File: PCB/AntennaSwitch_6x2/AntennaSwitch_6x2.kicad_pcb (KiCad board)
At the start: 2 copper layers, 100 x 100 mm, 160 parts, among them J1 Conn_01x08, J2 Conn_01x08, J3 Conn_01x08, J4 HR913550A, J5 SWD, J6 485, J7 12VDC, J8 Conn_01x01, Q1 2N7002K, SW1 LOAD, SW2 SRBV170501, SW3 SRBV170501, SW4 M/R, SW5 RESET, U1 74HC238, U10 74HC148, U11 74HC148, U12 4511, U13 4511, U14 Blue 0.59'', U15 Blue 0.59'', U16 STM32F030F4Px, U17 MAX485E, U18 CH395Q, U19 AZ1117-1.8, U2 74HC573, U20 SY8303, U3 74HC573, U4 74HC238, U5 74HC00, U6 74HC00, U7 74HC00, U8 74HC04, U9 TLC555, Y1 30MHz

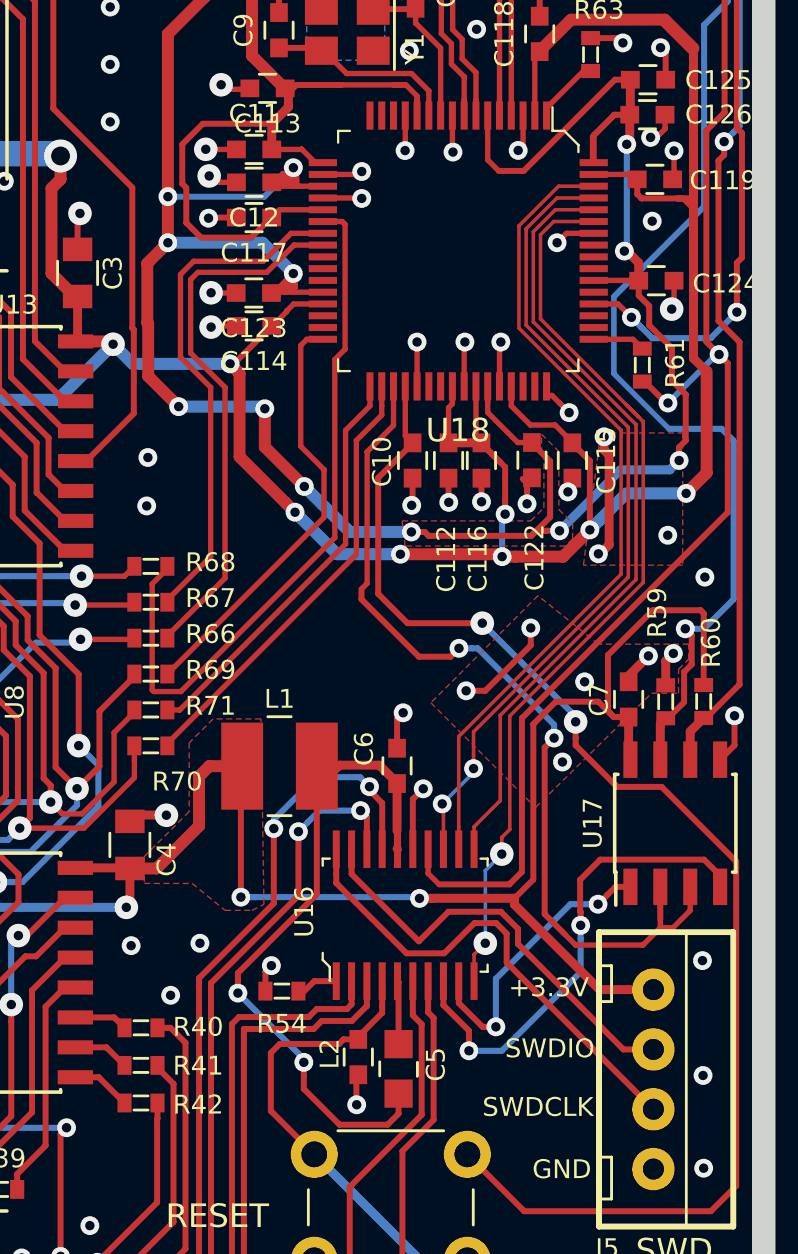
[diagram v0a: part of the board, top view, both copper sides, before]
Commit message: Relay Board SCH
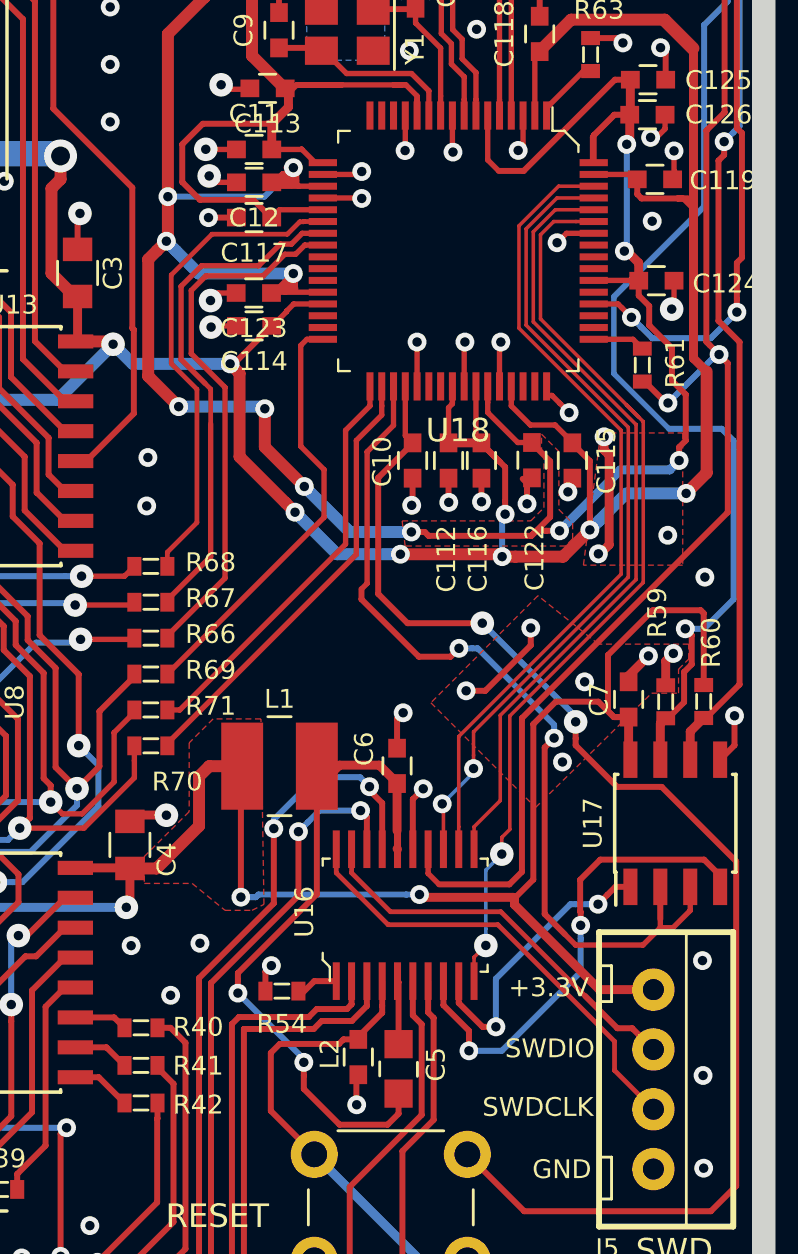
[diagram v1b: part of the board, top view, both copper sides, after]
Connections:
- net GND renamed chasis
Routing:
- net Net-(R68-Pad2): track 30.4 -> 20.7 mm
- net +3V3: track 887.9 -> 886.3 mm
- net /Remote/SWDIO: track 18.4 -> 16.9 mm
- net /Remote/SWCLK: track 20.7 -> 19.3 mm
- net chasis: track 201.3 -> 201.5 mm, vias 184 -> 185
- net +12V: vias 0 -> 3
- net (no net): vias 5 -> 1
- added copper zone on F.Cu, net GND
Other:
- net class CHASIS added: clearance 0.508, trace_width 0.2032, via_dia 0.8, via_drill 0.4
